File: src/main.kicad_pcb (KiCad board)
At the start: 4 copper layers, 54 parts, among them P301 CONN_01X15, P302 CONN_01X03, P501 CONN_01X07, Q501 MMBT3904, Q502 MMBT3904, U301 LM741, U302 DG444, U303 LM741, U304 LM741, U305 LM311N, U501 LM741, U502 LM741, U503 2DW232

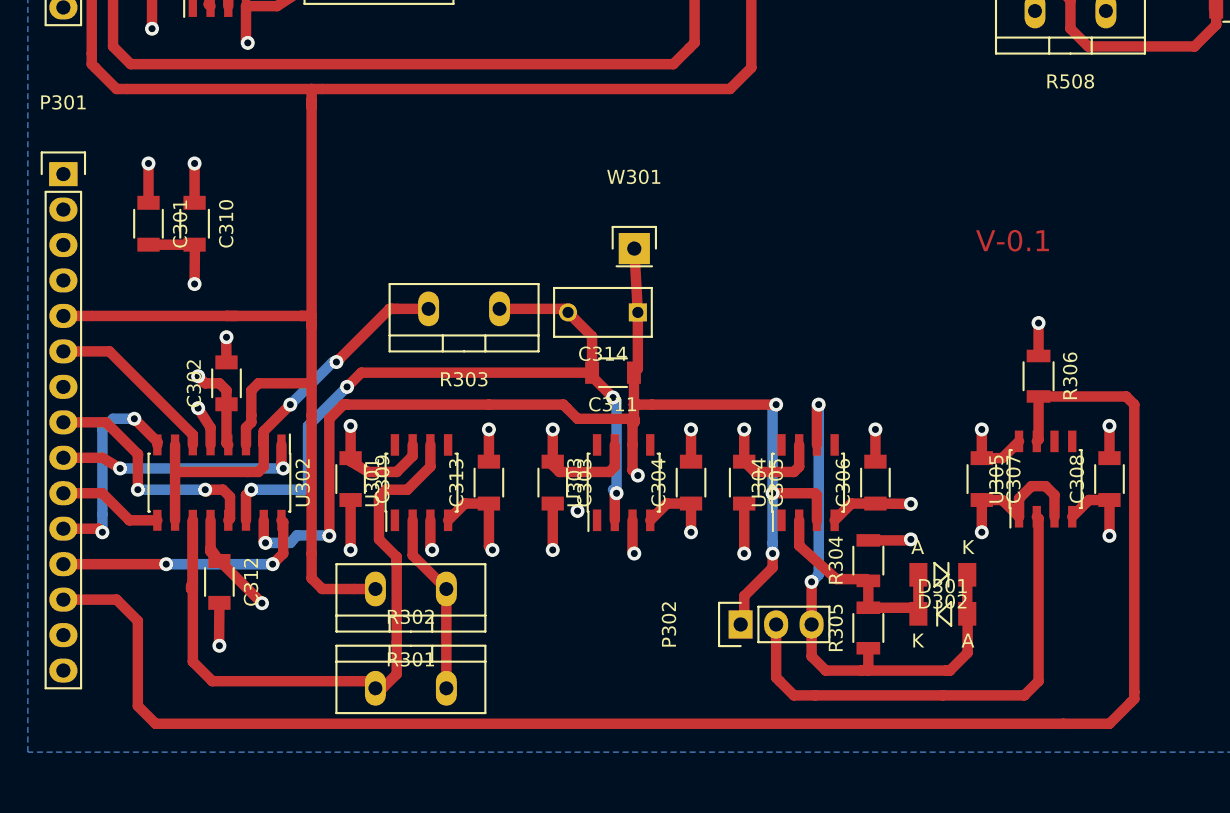
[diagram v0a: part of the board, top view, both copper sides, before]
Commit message: update
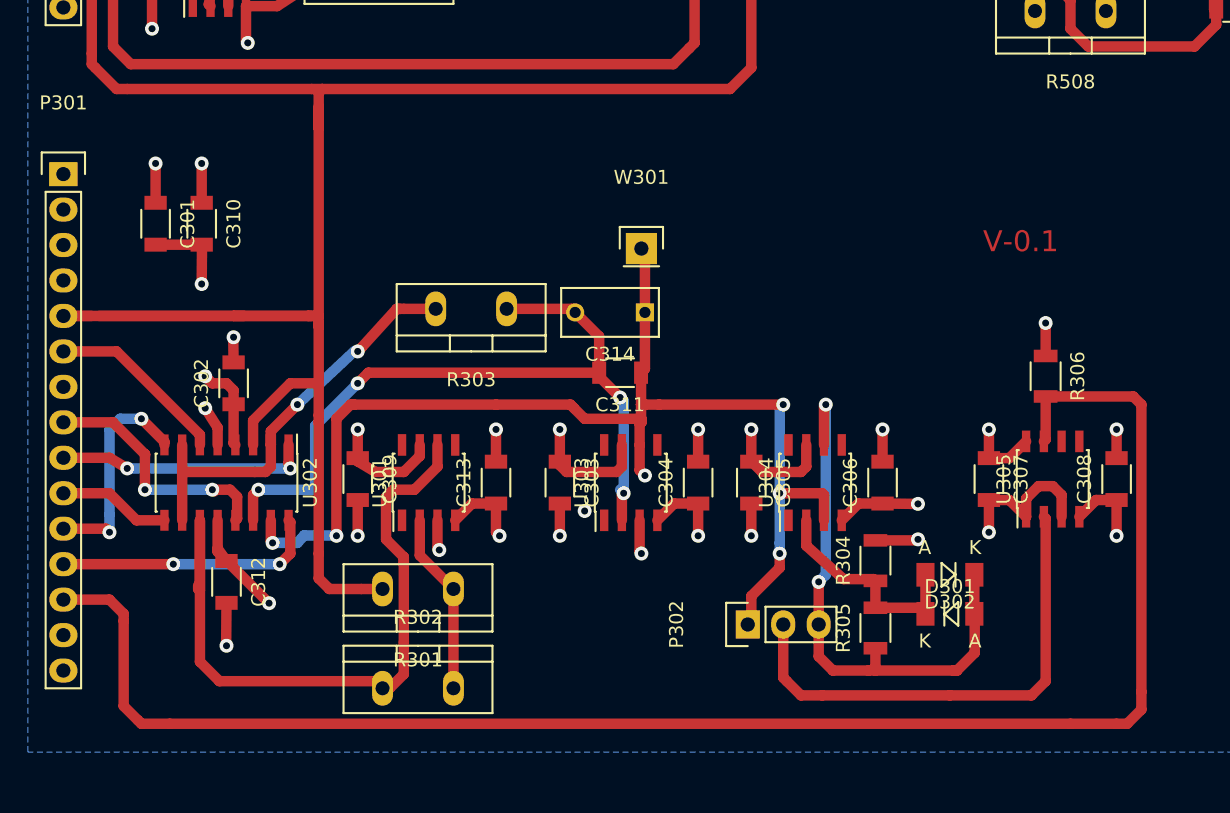
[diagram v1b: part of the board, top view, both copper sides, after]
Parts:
- moved C305 0.51 mm to (93.2, 85.1)
- moved C307 0.51 mm to (110.2, 84.8)
- moved C313 0.51 mm to (74.9, 85.1)
- moved R304 0.51 mm to (102.1, 90.7)
- moved R305 0.51 mm to (102.1, 95.5)
- moved U304 0.51 mm to (97.8, 85.1)
- moved U305 0.51 mm to (114.8, 84.8)
- moved C301 0.51 mm to (50.5, 66.5)
- moved C302 0.51 mm to (56.1, 78.0)
- moved C303 0.51 mm to (79.5, 85.1)
- moved C304 0.51 mm to (89.4, 85.1)
- moved C306 0.51 mm to (102.6, 85.1)
- moved C308 0.51 mm to (119.4, 84.8)
- moved C309 0.51 mm to (65.0, 84.8)
- moved C310 0.51 mm to (53.8, 66.5)
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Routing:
- net REF: track 192.0 -> 210.4 mm
- net 0V: track 76.4 -> 72.8 mm
- net -VE: track 49.8 -> 49.0 mm
- net TRIGGER: track 116.1 -> 116.9 mm
